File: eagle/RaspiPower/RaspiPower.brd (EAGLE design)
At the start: 50 x 33.5 mm, 26 parts, among them J5 AVR_SPI_PROG_3X2PTH, K1 4052

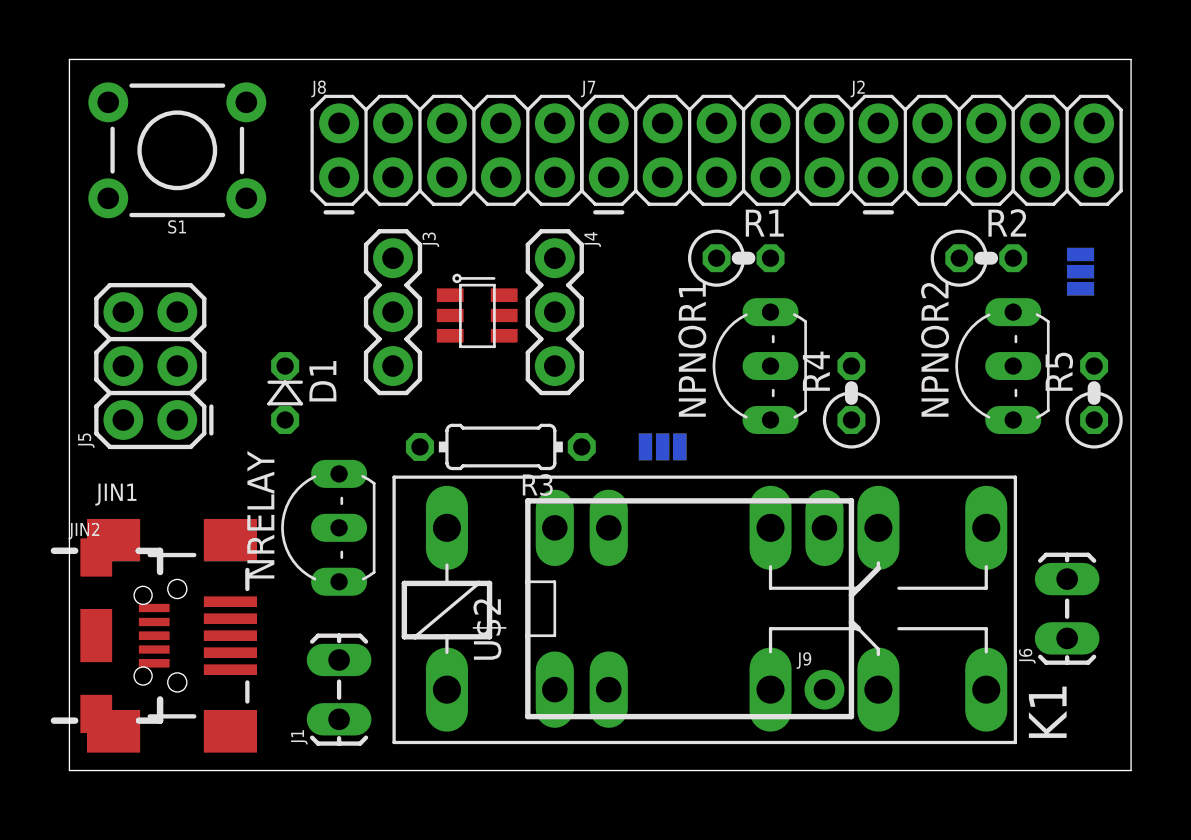
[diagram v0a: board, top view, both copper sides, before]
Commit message: Last changes before routing, added power LED
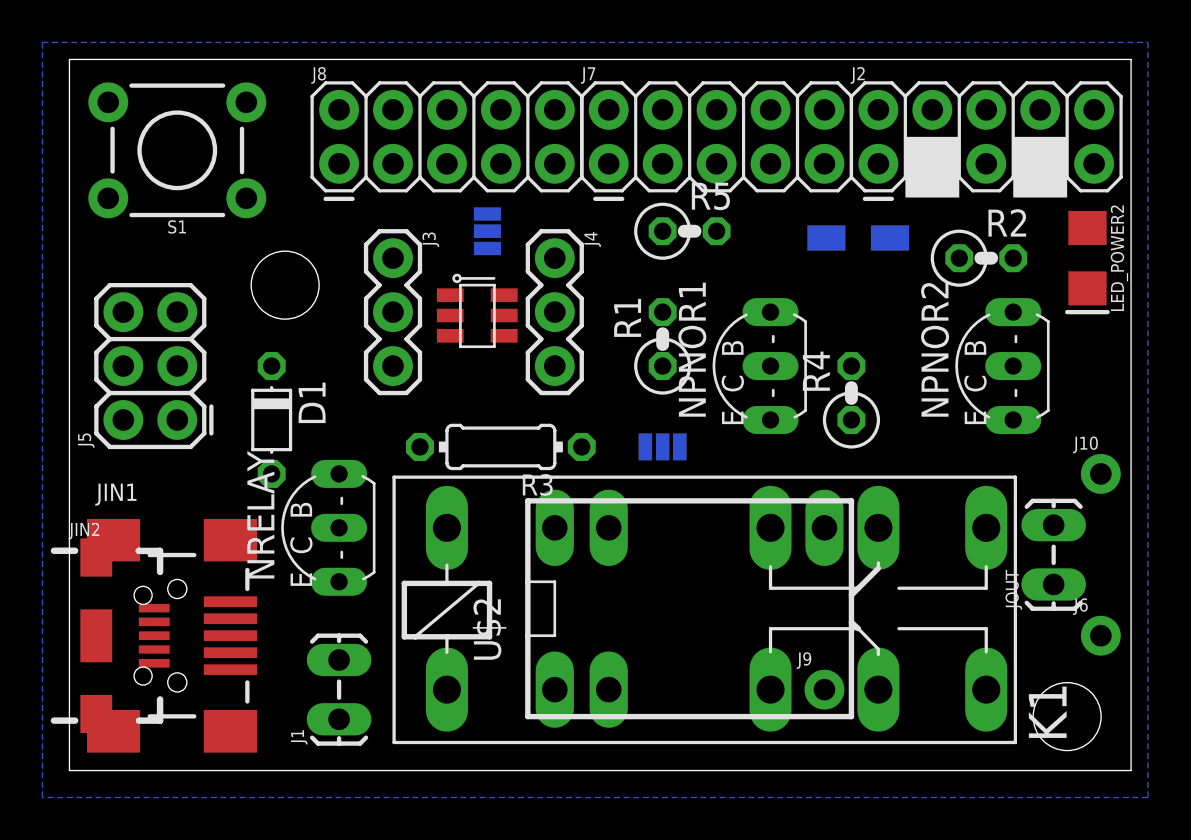
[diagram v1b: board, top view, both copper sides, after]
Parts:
- added J10: (no value), SparkFun-Connectors:1X01_NO_SILK
- added JOUT: (no value), SparkFun-Connectors:1X02_LOCK_LONGPADS
- added LED_POWER2: (no value), SparkFun-LED:FKIT-LED-1206
- added R6: 1k, resistor:R1206W
- D1: device diode:D-2.5 -> diode:D-5
- J6: device SparkFun-Connectors:1X02_LOCK_LONGPADS -> SparkFun-Connectors:1X01_NO_SILK
- R4, R5: value 1k -> 10k
- moved JP1 28.0 mm to (19.7, 25.4)
- moved R5 20.5 mm to (29.2, 25.4), turned to 0 degrees
- moved R1 5.39 mm to (27.9, 20.3), turned to 90 degrees
- moved J6 1.59 mm to (48.6, 6.35), turned to 0 degrees
- moved D1 1.42 mm to (9.53, 16.5)
- moved J2 0.63 mm to (38.1, 28.6)
- moved J7 0.63 mm to (25.4, 28.6)
- moved J8 0.63 mm to (12.7, 28.6)
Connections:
- new net N$1: LED_POWER2.A, R6.1
- net GND: now also JOUT.2, LED_POWER2.C; no longer J6.2
- net N$3: now also JOUT.1; no longer J6.1
- net VCC: now also R6.2
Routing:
- added copper zone on layer 16, net GND
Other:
- board text added: "E C B"
